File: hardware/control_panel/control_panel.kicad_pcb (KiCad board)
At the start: 2 copper layers, 13.5 x 21.5 mm, 2 parts, among them SW1 RotaryEncoder_Switch_MP

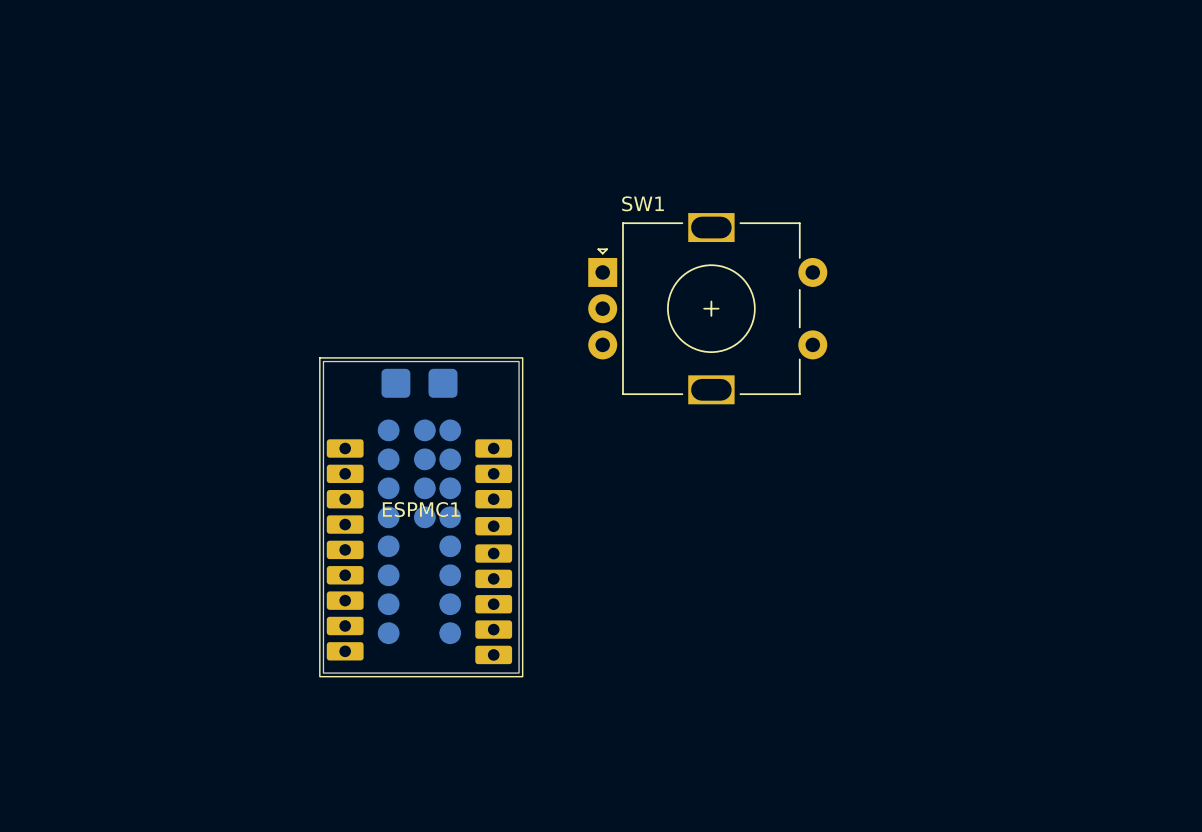
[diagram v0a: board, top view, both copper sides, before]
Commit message: KiCad updates and EC11 to TWT
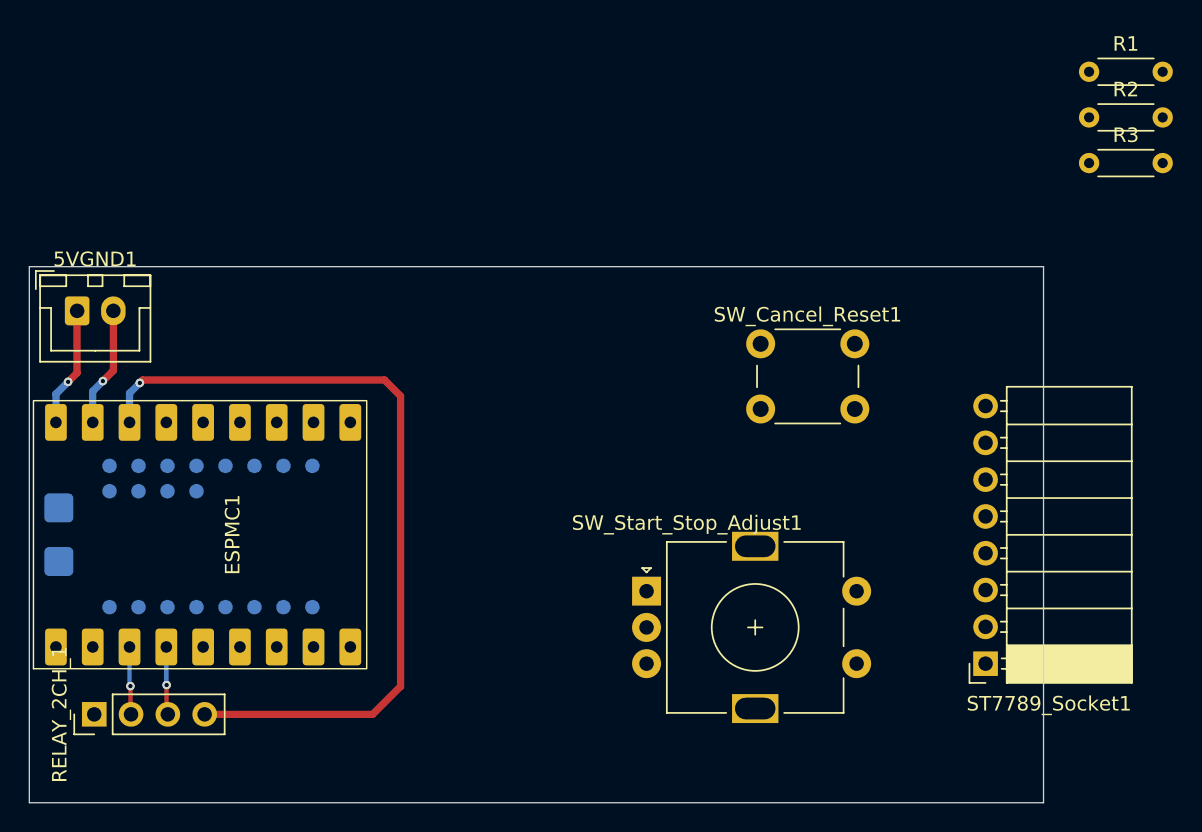
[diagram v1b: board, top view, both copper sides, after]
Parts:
- removed SW1: RotaryEncoder_Switch_MP, Rotary_Encoder:RotaryEncoder_Alps_EC11E-Switch_Vertical_H20mm
- added 5VGND1: Conn_01x02_Pin, Connector_JST:JST_XH_B2B-XH-A_1x02_P2.50mm_Vertical, F.Cu at (53.3, 53.0)
- added R1: 10k, Resistor_THT:R_Axial_DIN0204_L3.6mm_D1.6mm_P5.08mm_Horizontal, F.Cu at (123.1, 36.5)
- added R2: 10k, Resistor_THT:R_Axial_DIN0204_L3.6mm_D1.6mm_P5.08mm_Horizontal, F.Cu at (123.1, 39.7)
- added R3: 10k, Resistor_THT:R_Axial_DIN0204_L3.6mm_D1.6mm_P5.08mm_Horizontal, F.Cu at (123.1, 42.9)
- added RELAY_2CH_1: Conn_01x04_Pin, Connector_PinHeader_2.54mm:PinHeader_1x04_P2.54mm_Vertical, F.Cu at (54.5, 80.9)
- added ST7789_Socket1: Conn_01x08_Socket, Connector_PinSocket_2.54mm:PinSocket_1x08_P2.54mm_Horizontal, F.Cu at (116.0, 77.4)
- added SW_Cancel_Reset1: SW_Push, Button_Switch_THT:SW_PUSH_6mm_H8.5mm, F.Cu at (100.5, 55.3)
- added SW_Start_Stop_Adjust1: RotaryEncoder_Switch_MP, Rotary_Encoder:RotaryEncoder_Alps_EC11E-Switch_Vertical_H20mm, F.Cu at (92.6, 72.4)
- moved ESPMC1 12.6 mm to (64.5, 68.5), turned to 90 degrees
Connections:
- ESPMC1 pad 1: unconnected-(ESPMC1-GP1-Pad1) -> /IN1_FAN
- ESPMC1 pad 10: unconnected-(ESPMC1-GP10-Pad10) -> /LCD_RST
- ESPMC1 pad 11: unconnected-(ESPMC1-GP11-Pad11) -> /LCD_SDA
- ESPMC1 pad 12: unconnected-(ESPMC1-GP12-Pad12) -> /LCD_SCL
- ESPMC1 pad 2: unconnected-(ESPMC1-GP2-Pad2) -> /IN2_LEDS
- ESPMC1 pad 3V3: unconnected-(ESPMC1-3V3(OUT)-Pad3V3) -> /3V3+
- ESPMC1 pad 4: unconnected-(ESPMC1-GP4-Pad4) -> Net-(ESPMC1-GP4)
- ESPMC1 pad 5: unconnected-(ESPMC1-GP5-Pad5) -> Net-(ESPMC1-GP5)
- ESPMC1 pad 5V: unconnected-(ESPMC1-Pad5V) -> Net-(5VGND1-Pin_1)
- ESPMC1 pad 6: unconnected-(ESPMC1-GP6-Pad6) -> Net-(ESPMC1-GP6)
- ESPMC1 pad 7: unconnected-(ESPMC1-GP7-Pad7) -> Net-(ESPMC1-GP7)
- ESPMC1 pad 8: unconnected-(ESPMC1-GP8-Pad8) -> /LCD_BL
- ESPMC1 pad 9: unconnected-(ESPMC1-GP9-Pad9) -> /LCD_DC
- ESPMC1 pad GND: unconnected-(ESPMC1-PadGND) -> GND
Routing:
- net /3V3+: track 0.00 -> 55.9 mm, vias 0 -> 1
- net Net-(5VGND1-Pin_1): track 0.00 -> 8.31 mm, vias 0 -> 1
- net GND: track 0.00 -> 8.29 mm, vias 0 -> 1
- net /IN2_LEDS: track 0.00 -> 4.81 mm, vias 0 -> 1
- net /IN1_FAN: track 0.00 -> 4.76 mm, vias 0 -> 1
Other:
- board size 13.5 x 21.5 mm -> 70 x 37 mm
